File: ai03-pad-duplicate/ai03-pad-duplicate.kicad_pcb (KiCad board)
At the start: 2 copper layers, 68.7 x 38.1 mm, 24 parts, among them SW1 SW_Push, U1 ATmega32U4-AU, Y1 16MHz

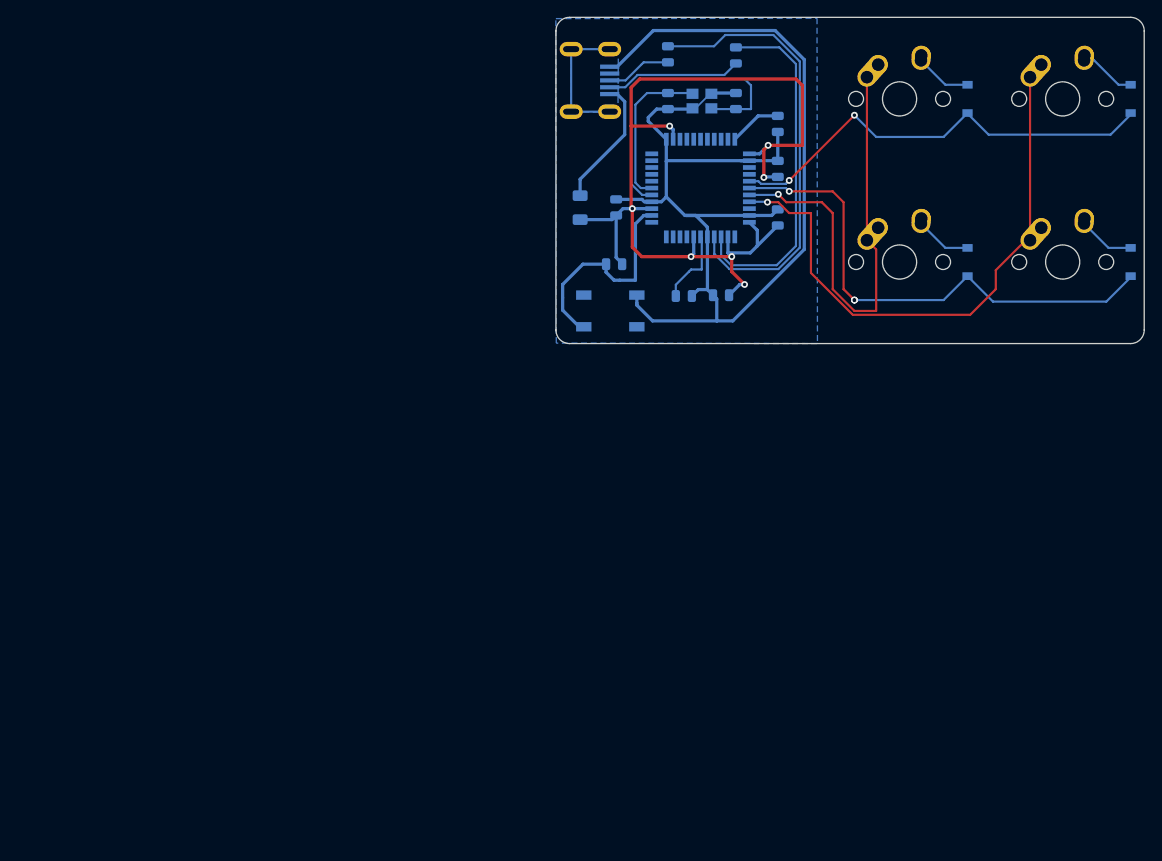
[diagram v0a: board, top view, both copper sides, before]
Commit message: Complete the PCB
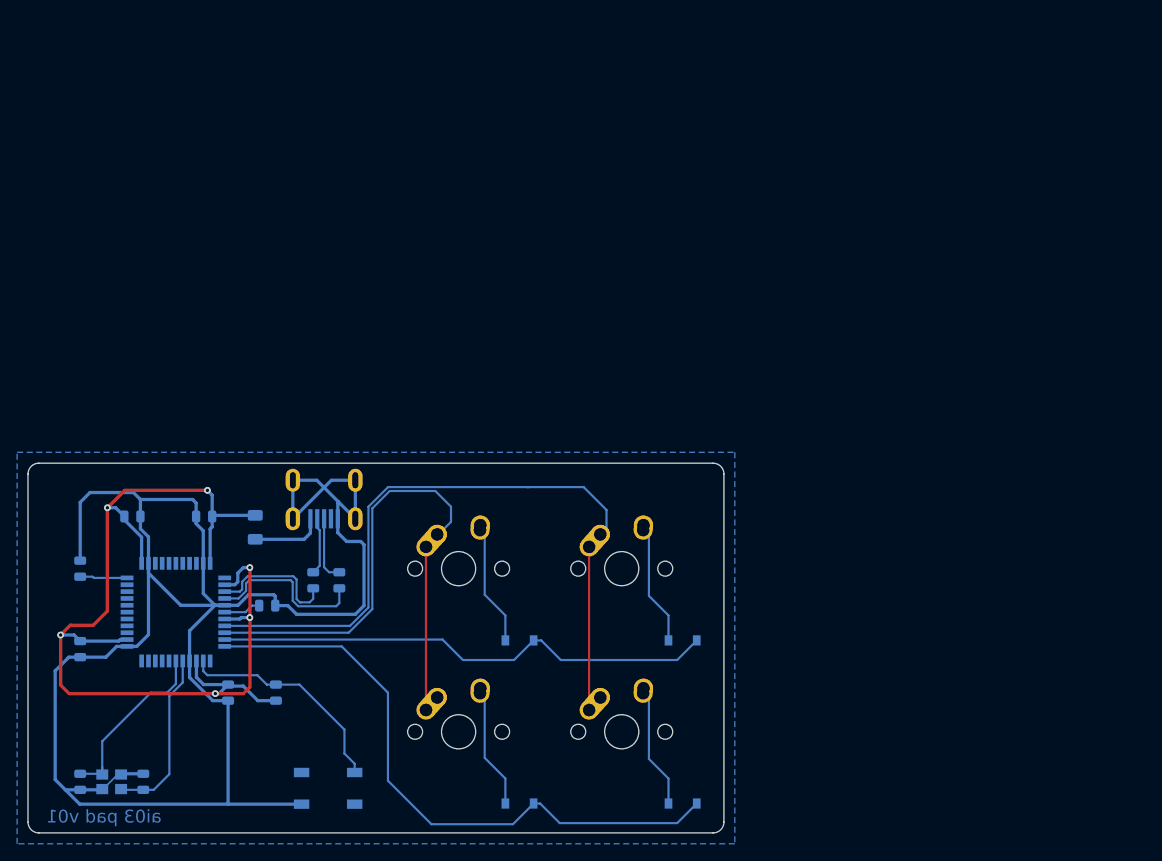
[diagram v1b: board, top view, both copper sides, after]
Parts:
- moved C2 105.4 mm to (77.0, 171.8), turned to 90 degrees
- moved Y1 105.2 mm to (73.3, 171.8)
- moved C1 105.0 mm to (69.6, 171.8), turned to -90 degrees
- moved R4 96.6 mm to (69.6, 146.9), turned to 90 degrees
- moved C6 85.6 mm to (75.7, 140.8), turned to 0 degrees
- moved C5 85.5 mm to (69.6, 156.3), turned to -90 degrees
- moved D1 82.1 mm to (120.9, 155.3), turned to 180 degrees
- moved D2 82.1 mm to (120.9, 174.4), turned to 180 degrees
- moved D3 82.1 mm to (140.0, 155.3), turned to 180 degrees
- moved D4 82.1 mm to (140.0, 174.4), turned to 180 degrees
- moved U1 78.8 mm to (80.8, 152.0), turned to 180 degrees
- moved R1 78.7 mm to (96.8, 148.3), turned to -90 degrees
- moved C7 75.5 mm to (84.1, 140.8), turned to 180 degrees
- moved MX1 75.2 mm to (113.8, 146.9)
- moved MX2 75.2 mm to (113.8, 166.0)
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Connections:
- C1 pad 1: GND -> Net-(C1-Pad1)
- C1 pad 2: Net-(C1-Pad2) -> GND
- C2 pad 1: GND -> Net-(C2-Pad1)
- C2 pad 2: Net-(C2-Pad2) -> GND
- U1 pad 10: Net-(U1-Pad10) -> ROW0
- U1 pad 11: Net-(U1-Pad11) -> ROW1
- U1 pad 16: Net-(C2-Pad2) -> Net-(C2-Pad1)
- U1 pad 17: Net-(C1-Pad2) -> Net-(C1-Pad1)
- U1 pad 38: ROW0 -> Net-(U1-Pad38)
- U1 pad 39: ROW1 -> Net-(U1-Pad39)
- U1 pad 40: COL0 -> Net-(U1-Pad40)
- U1 pad 41: COL1 -> Net-(U1-Pad41)
- U1 pad 8: Net-(U1-Pad8) -> COL1
- U1 pad 9: Net-(U1-Pad9) -> COL0
- USB1 pad 6: Net-(USB1-Pad6) -> GND
- Y1 pad 1: Net-(C2-Pad2) -> Net-(C2-Pad1)
- Y1 pad 3: Net-(C1-Pad2) -> Net-(C1-Pad1)
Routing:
- net GND: track 149.1 -> 216.2 mm
- net Net-(C2-Pad2): track 36.4 -> 0.00 mm
- net Net-(R2-Pad1): track 52.7 -> 19.2 mm
- net Net-(R1-Pad2): track 41.4 -> 15.6 mm
- net Net-(C1-Pad1): track 0.00 -> 21.4 mm
- net Net-(C2-Pad1): track 0.00 -> 20.3 mm
- net Net-(C1-Pad2): track 18.5 -> 0.00 mm
- net COL1: track 66.3 -> 83.8 mm, vias 1 -> 0
- net Net-(USB1-Pad6): track 16.3 -> 0.00 mm
- net ROW1: track 59.6 -> 72.7 mm, vias 3 -> 0
- net +5V: track 113.2 -> 126.3 mm, vias 7 -> 6
- net COL0: track 53.4 -> 65.9 mm, vias 1 -> 0
- net D-: track 15.9 -> 6.68 mm
- net Net-(D2-Pad2): track 6.62 -> 14.1 mm
- net Net-(D1-Pad2): track 6.62 -> 14.1 mm
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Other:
- board size 68.7 x 38.1 mm -> 81.3 x 43.2 mm
- board text added: "ai03 pad v01"
